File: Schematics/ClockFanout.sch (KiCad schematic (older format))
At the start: 20 parts, among them CN401 COAX, CN402 COAX, CN405 COAX, CN406 COAX, U401 NB3L553

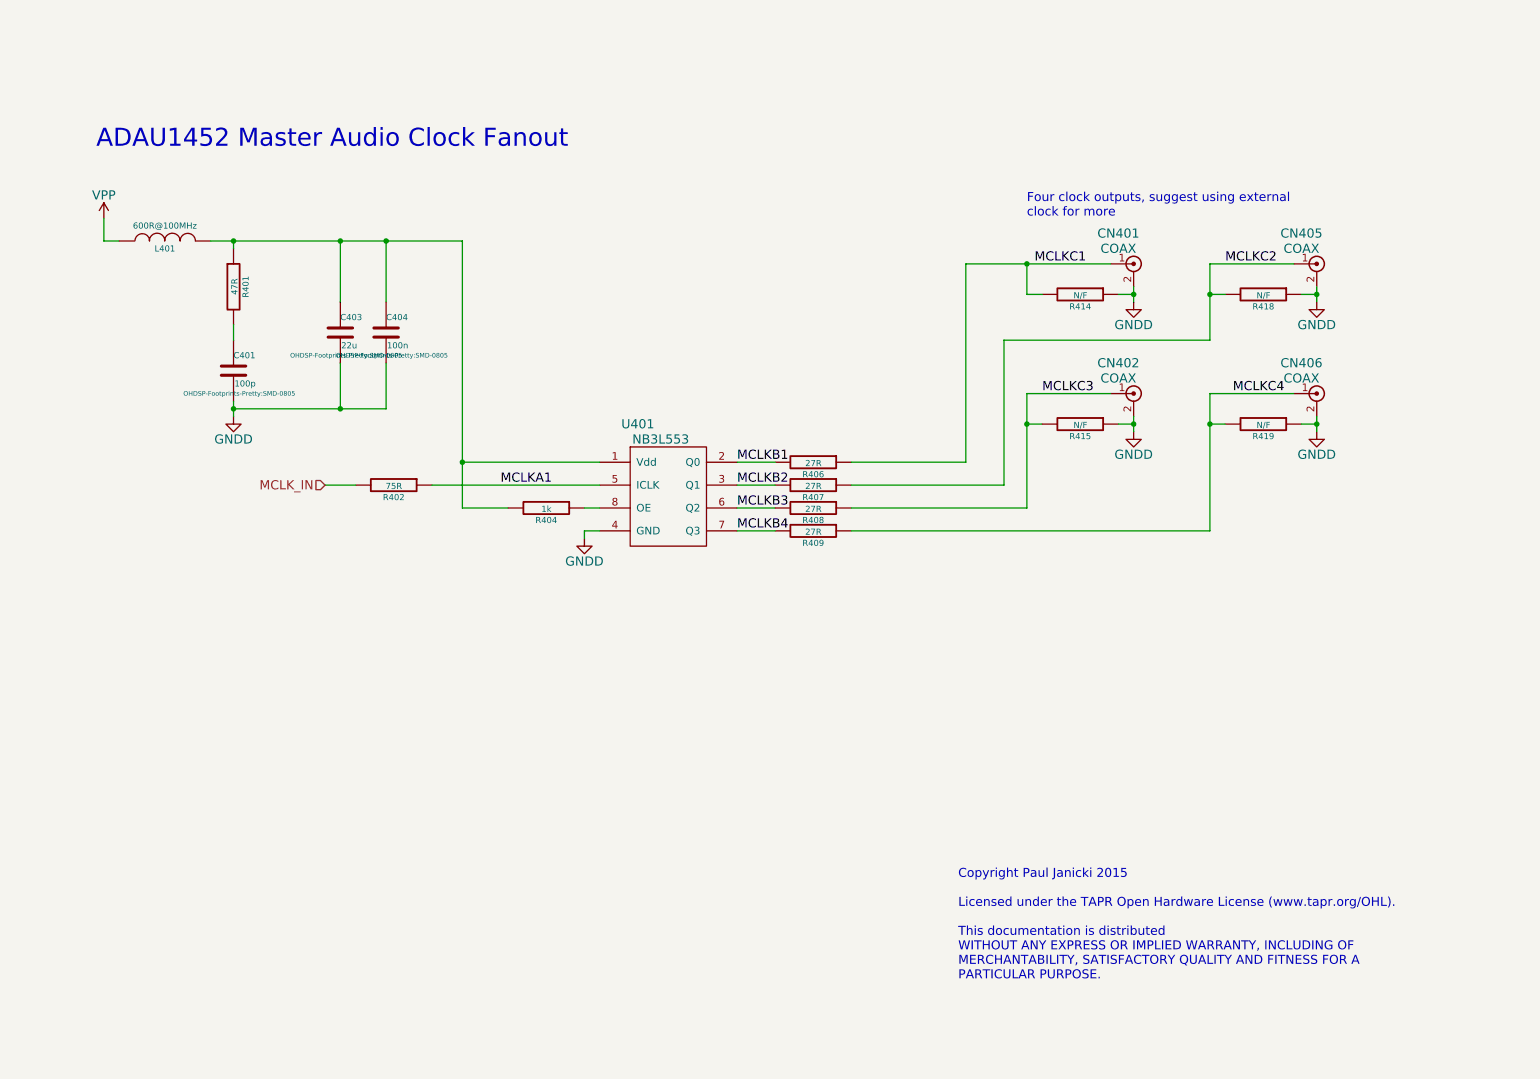
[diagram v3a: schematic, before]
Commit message: WIP
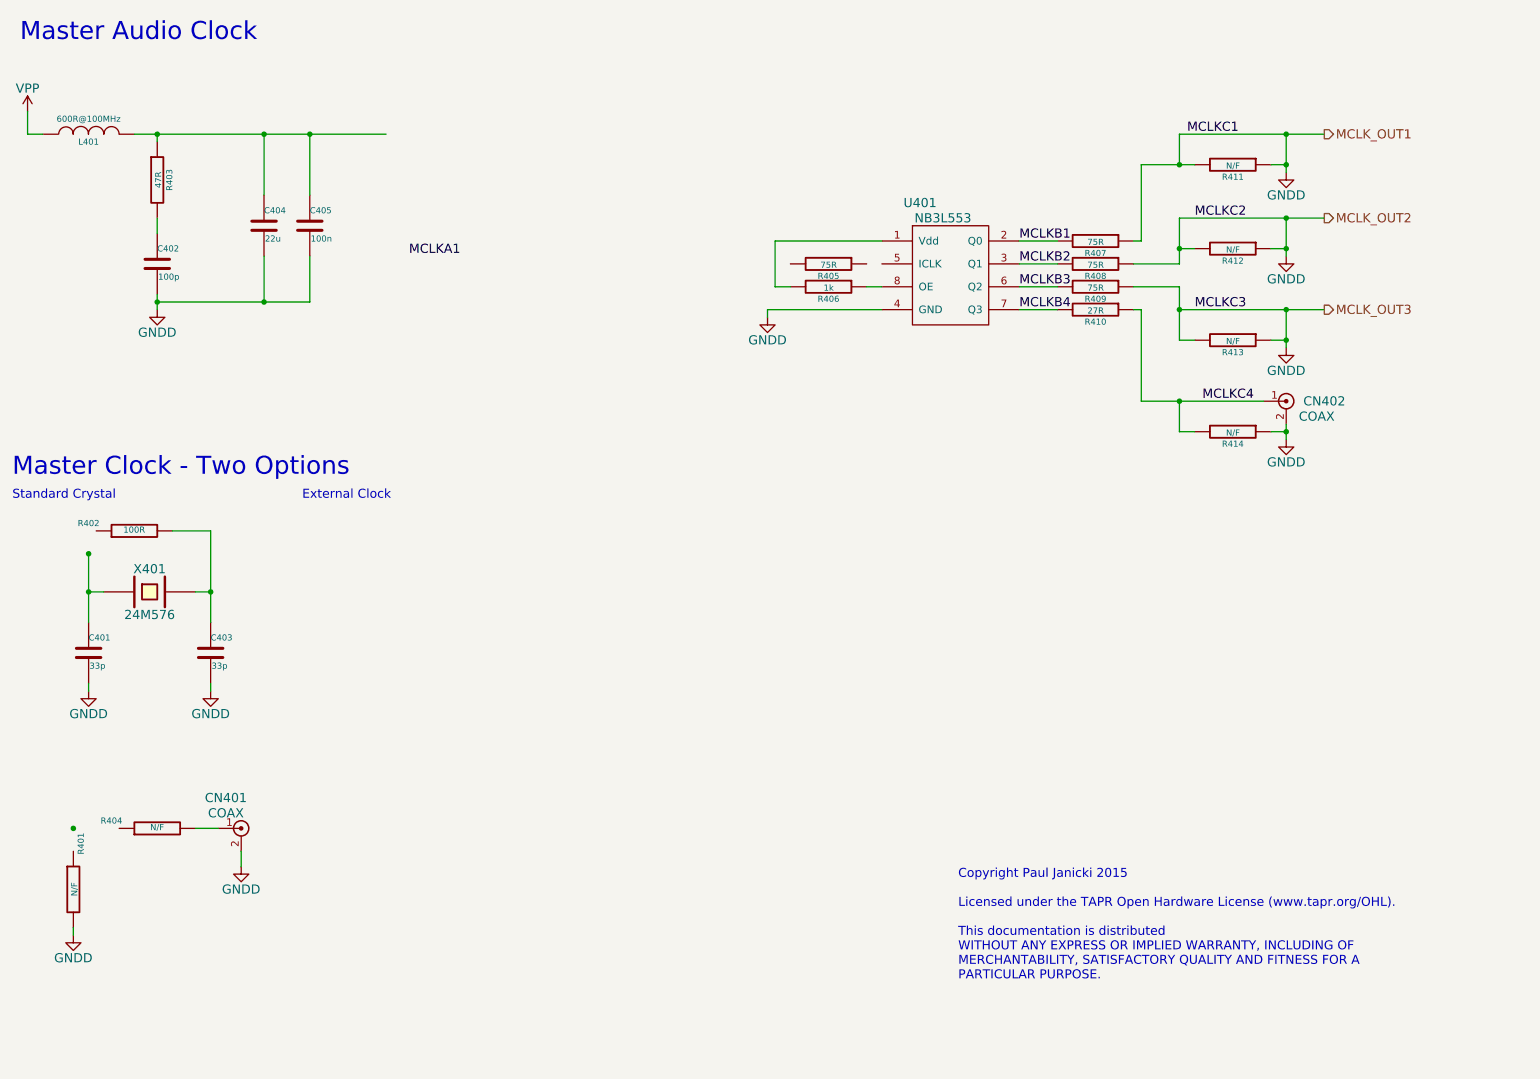
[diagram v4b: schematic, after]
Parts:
- removed CN402, CN405: COAX, OHDSP-Footprints-Pretty:CONN-RF-UFL, symbol COAX
- added C401, C403: 33p, symbol C
- added R401, R404: N/F, symbol R
- added R402: 100R, symbol R
- added X401: 24M576, symbol CRYSTAL
- C402: renamed from C401; footprint OHDSP-Footprints-Pretty:SMD-0805 -> (none)
- C404: renamed from C403; footprint OHDSP-Footprints-Pretty:SMD-0805 -> (none)
- C405: renamed from C404; footprint OHDSP-Footprints-Pretty:SMD-0805 -> (none)
- CN401: footprint OHDSP-Footprints-Pretty:CONN-RF-UFL -> (none)
- CN402: renamed from CN406; footprint OHDSP-Footprints-Pretty:CONN-RF-UFL -> (none)
- L401: footprint OHDSP-Footprints-Pretty:SMD-0805 -> (none)
- R403: renamed from R401; footprint OHDSP-Footprints-Pretty:SMD-0805 -> (none)
- R405: renamed from R402; footprint OHDSP-Footprints-Pretty:TH-RES-0W25 -> (none)
- R406: renamed from R404; footprint OHDSP-Footprints-Pretty:SMD-0805 -> (none)
- R407: renamed from R406; value 27R -> 75R; footprint OHDSP-Footprints-Pretty:SMD-0805 -> (none)
- R408: renamed from R407; value 27R -> 75R; footprint OHDSP-Footprints-Pretty:SMD-0805 -> (none)
- R409: renamed from R408; value 27R -> 75R; footprint OHDSP-Footprints-Pretty:SMD-0805 -> (none)
- R410: renamed from R409; footprint OHDSP-Footprints-Pretty:SMD-0805 -> (none)
- R411: renamed from R414; footprint OHDSP-Footprints-Pretty:SMD-0805 -> (none)
- R412: renamed from R418; footprint OHDSP-Footprints-Pretty:SMD-0805 -> (none)
- R413: renamed from R415; footprint OHDSP-Footprints-Pretty:SMD-0805 -> (none)
- R414: renamed from R419; footprint OHDSP-Footprints-Pretty:SMD-0805 -> (none)
- U401: footprint OHDSP-Footprints-Pretty:IC_SOIC_8 -> (none)
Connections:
- net MCLKC2 is gone; now on net GNDD: R408.1, R412.2
- net MCLKC3 is gone; now on net GNDD: R409.1, R413.2
- net GNDD: now also R407.1, R411.2, C401.2, C403.2, R401.2
- net MCLKA1: no longer R405.1, U401.5 (ICLK)
- net at C404.1, C405.1, L401.2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: no longer R406.2, U401.1 (Vdd)
- removed net MCLKC1: CN401.1, R407.1, R411.2
- net MCLK_IN: no longer names the net of R405.2
- new net: R406.2, U401.1 (Vdd)
- new net: C401.1, X401.1
- new net: C403.1, R402.2, X401.2
- new net: CN401.1, R404.2
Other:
- note added: "External Clock"
- note added: "Master Audio Clock"
- note added: "Master Clock - Two Options"
- note added: "Standard Crystal"
- note removed: "ADAU1452 Master Audio Clock Fanout"
- note removed: "Four clock outputs, suggest using external\nclock for more"
- moved on the sheet: C402, C404, C405, CN402, L401, R403, R405, R406, R407, R408, R409, R410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

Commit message: WIP
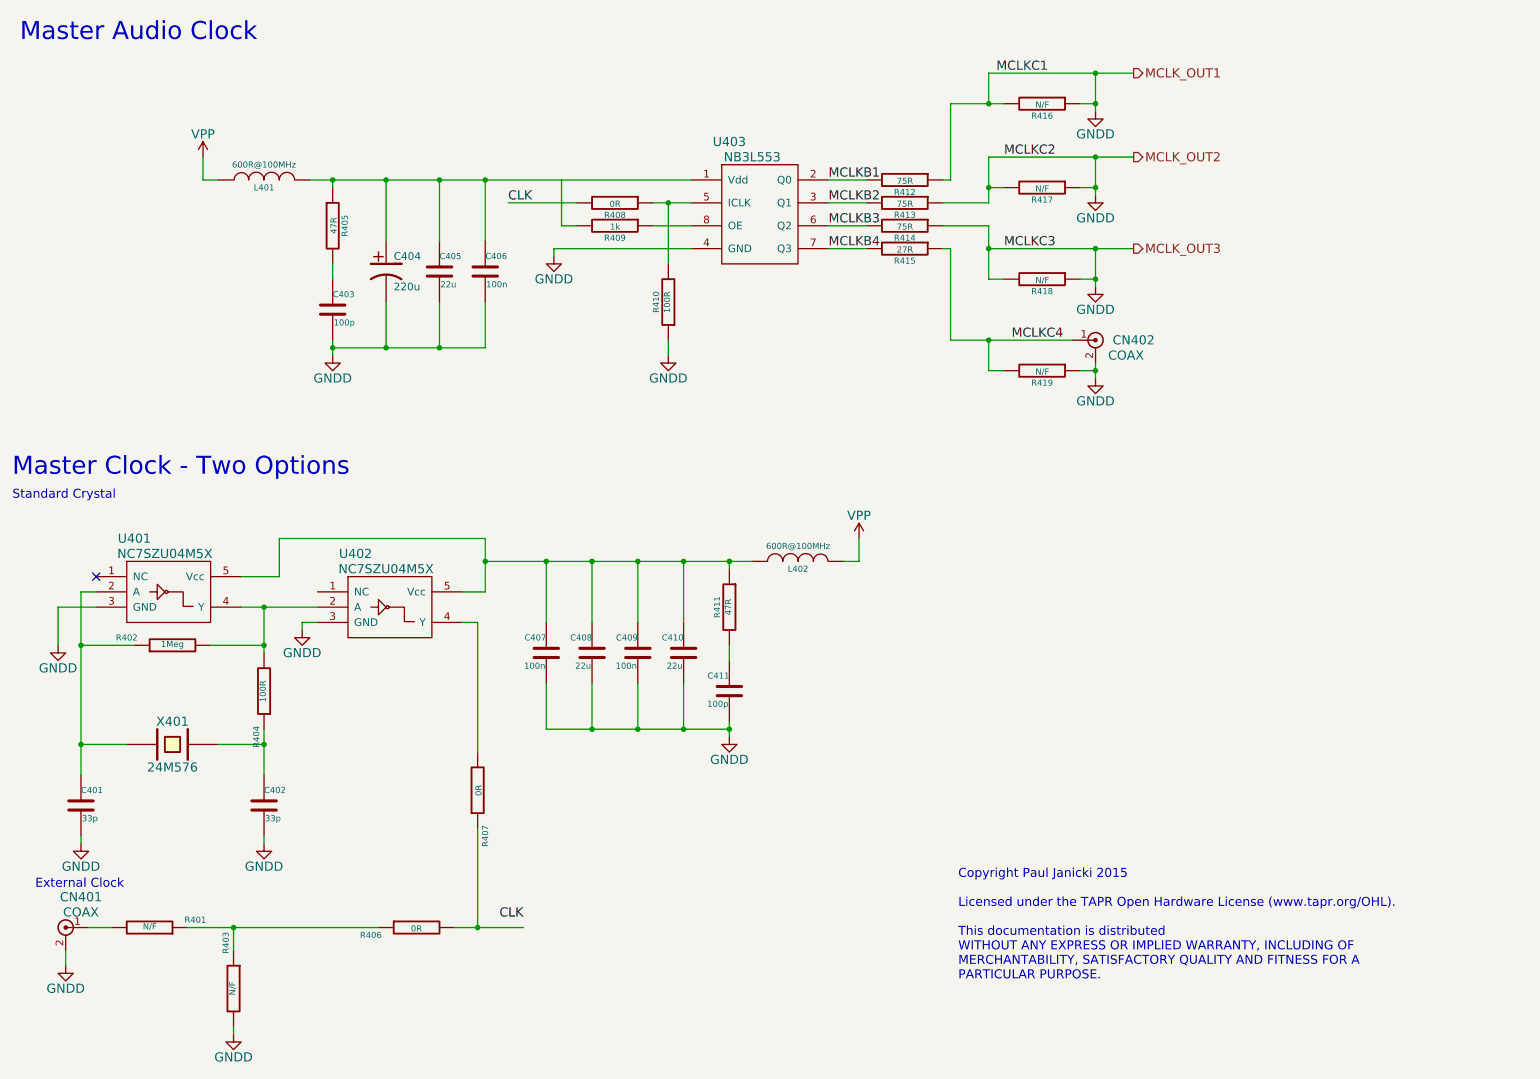
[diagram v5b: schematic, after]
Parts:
- added C404: 220u, OHDSP-Footprints-Pretty:SMD-0805, symbol CP1
- added C407, C409: 100n, symbol C
- added C408, C410: 22u, symbol C
- added C411: 100p, symbol C
- added L402: 600R@100MHz, symbol INDUCTOR
- added R402: 1Meg, OHDSP-Footprints-Pretty:SMD-0805, symbol R
- added R406, R407: 0R, OHDSP-Footprints-Pretty:SMD-0805, symbol R
- added R410: 100R, OHDSP-Footprints-Pretty:SMD-0805, symbol R
- added R411: 47R, OHDSP-Footprints-Pretty:SMD-0805, symbol R
- added U401: NC7SZU04M5X, OHDSP-Footprints-Pretty:IC_SOIC_8, symbol IC-LOGIC-NC7SZU04M5X
- added U402: NC7SZU04M5X, symbol IC-LOGIC-NC7SZU04M5X
- C401, L401: footprint (none) -> OHDSP-Footprints-Pretty:SMD-0805
- C402: renamed from C403; footprint (none) -> OHDSP-Footprints-Pretty:SMD-0805
- C403: renamed from C402; footprint (none) -> OHDSP-Footprints-Pretty:SMD-0805
- C405: renamed from C404; footprint (none) -> OHDSP-Footprints-Pretty:SMD-0805
- CN401, CN402: footprint (none) -> OHDSP-Footprints-Pretty:CONN-RF-UFL
- R401: renamed from R404; footprint (none) -> OHDSP-Footprints-Pretty:SMD-0805
- R403: renamed from R401; footprint (none) -> OHDSP-Footprints-Pretty:SMD-0805
- R404: renamed from R402; footprint (none) -> OHDSP-Footprints-Pretty:SMD-0805
- R405: renamed from R403; footprint (none) -> OHDSP-Footprints-Pretty:SMD-0805
- R408: renamed from R405; value 75R -> 0R; footprint (none) -> OHDSP-Footprints-Pretty:SMD-0805
- R409: renamed from R406; footprint (none) -> OHDSP-Footprints-Pretty:SMD-0805
- R412: renamed from R407; footprint (none) -> OHDSP-Footprints-Pretty:SMD-0805
- R413: renamed from R408; footprint (none) -> OHDSP-Footprints-Pretty:SMD-0805
- R414: renamed from R409; footprint (none) -> OHDSP-Footprints-Pretty:SMD-0805
- X401: footprint (none) -> OHDSP-Footprints-Pretty:XTAL_HC49_TH
- renumbered C405 to C406, R410 to R415, R411 to R416, R412 to R417, R413 to R418, R414 to R419, U401 to U403
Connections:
- net GNDD: now also C404.2, C407.2, C408.2, C409.2, C410.2, C411.2, R410.1, U401.3 (GND), U402.3 (GND)
- net VPP: now also L402.1
- net at U403.1 (Vdd): now also C405.1, C406.1, L401.2, R405.1, C404.1; no longer R409.2
- net at U403.5 (ICLK): now also R408.1, R410.2
- net CLK: now reaches R408.2
- net at C401.1, X401.1: now also R402.1, U401.2 (A)
- net at C402.1, X401.2: now also R404.1; no longer R404.2
- net at R401.1: now also R403.1, R406.1
- new net: R402.2, R404.2, U401.4 (Y), U402.2 (A)
- new net: C407.1, C408.1, C409.1, C410.1, L402.2, R411.1, U401.5 (Vcc), U402.5 (Vcc)
- new net: R407.2, U402.4 (Y)
- new net: C411.1, R411.2
- new net: R406.2, R407.1
- no-connect marks 0 -> 1
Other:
- moved on the sheet: C401, C402, C403, C405, C406, CN401, CN402, L401, R401, R403, R404, R405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
